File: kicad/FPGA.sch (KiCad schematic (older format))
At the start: 43 parts, among them U11 tx176, U3 MCP4725, X1 Stiftleiste_2x10Pm_R2.54

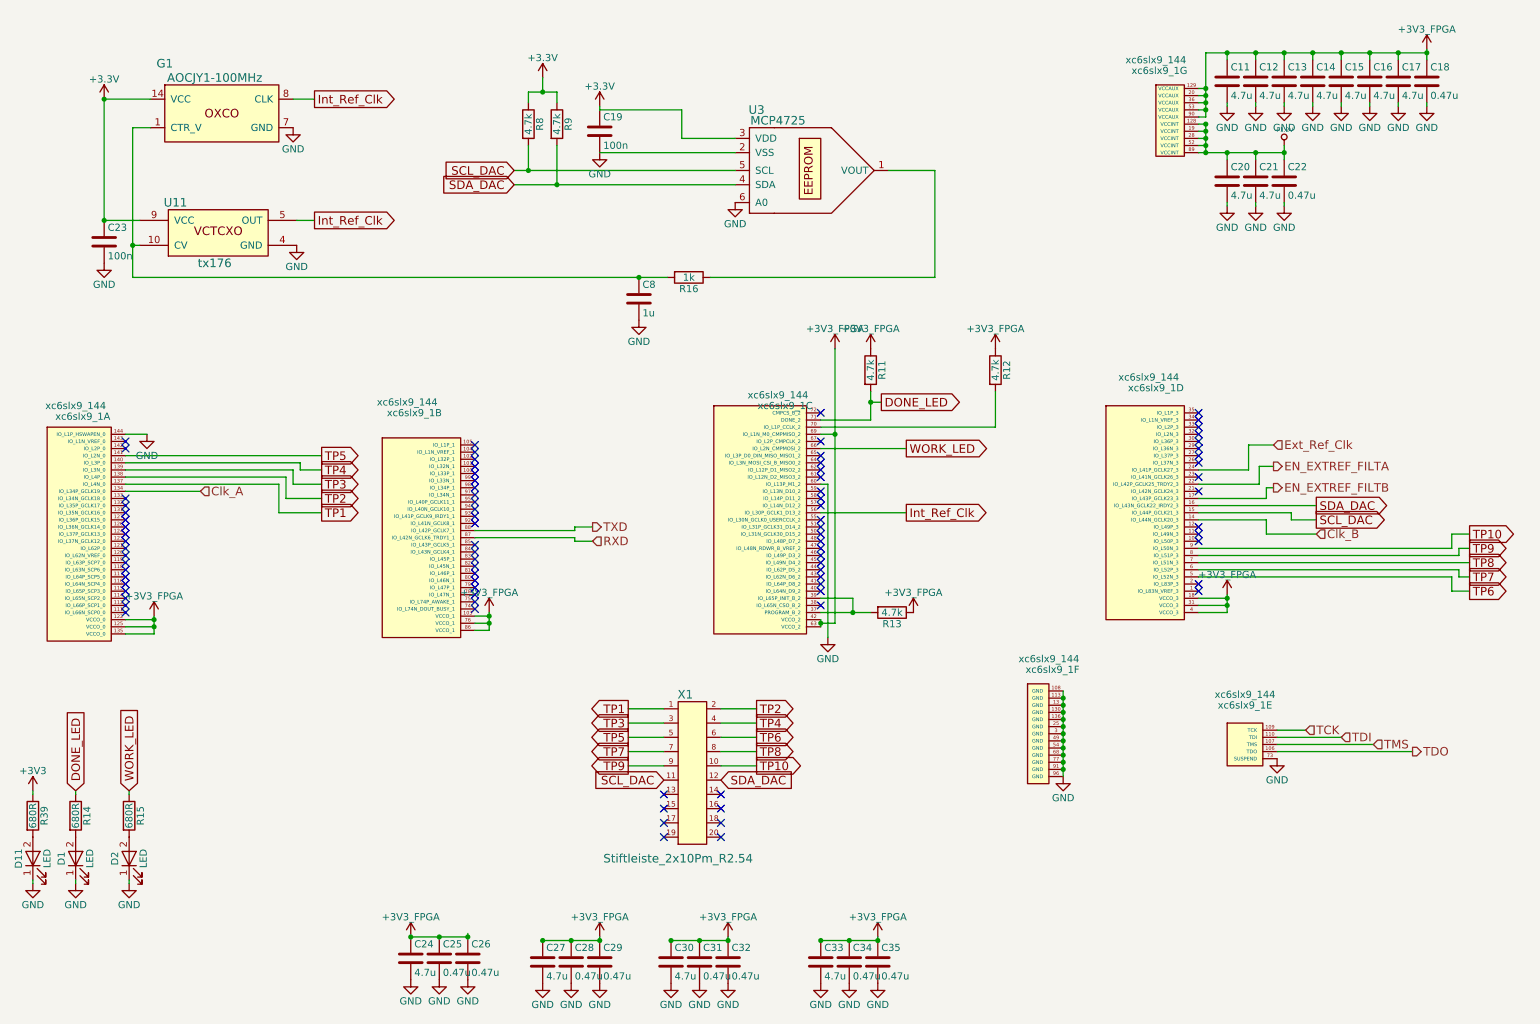
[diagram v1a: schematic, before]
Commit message: some small schematic and layout changes [completed]
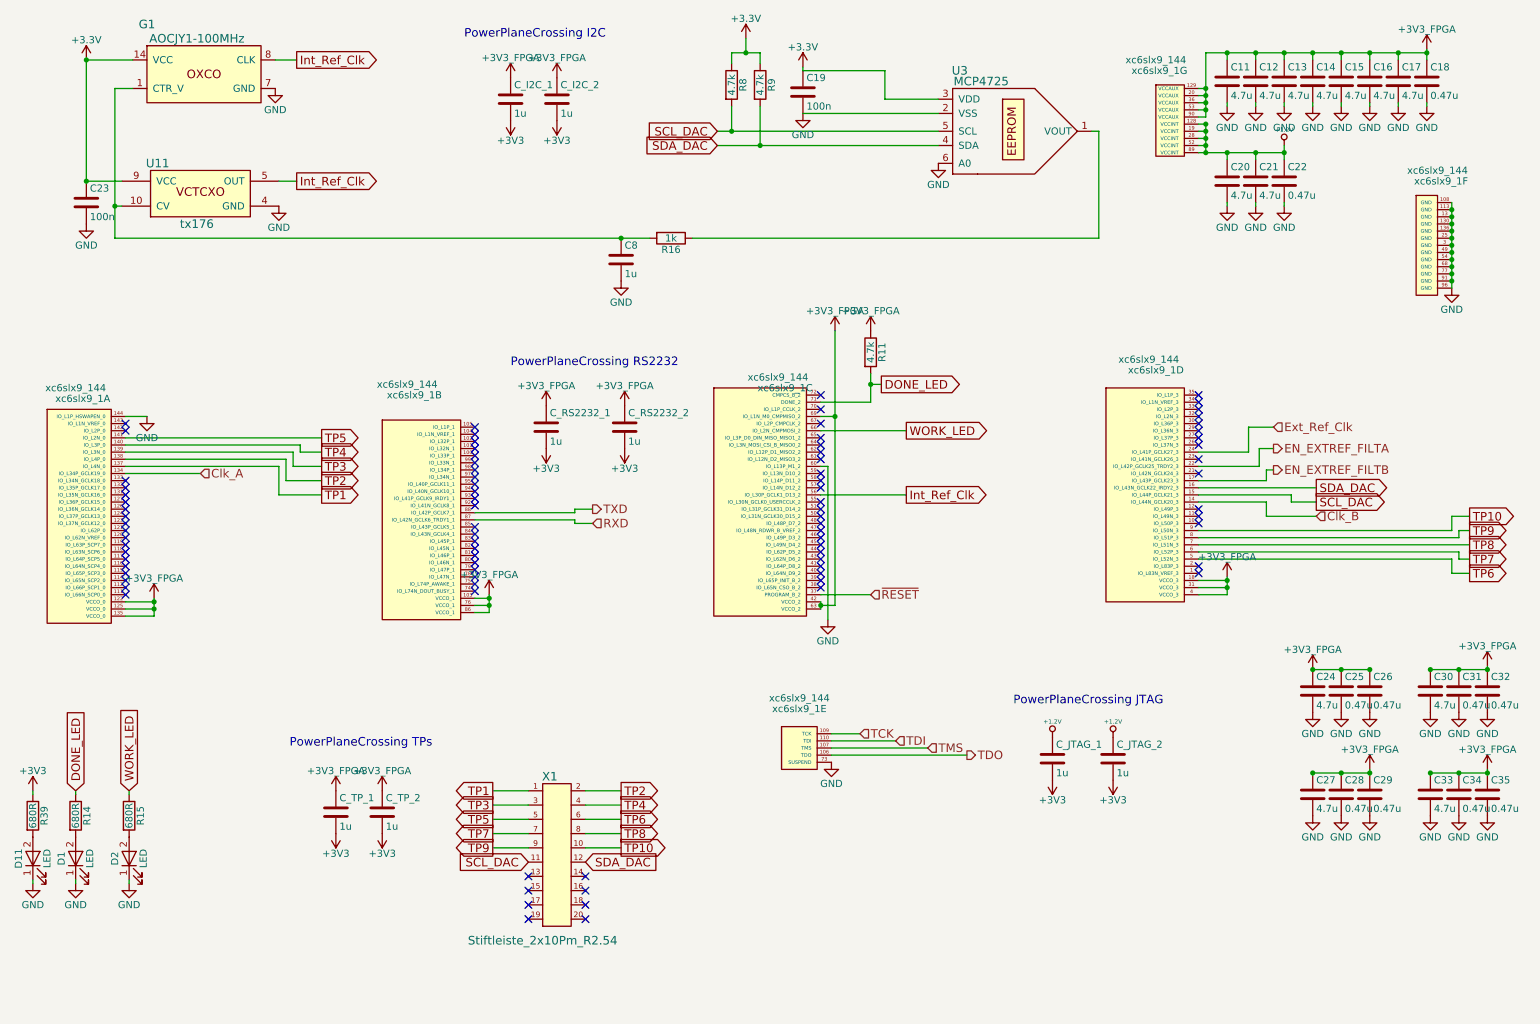
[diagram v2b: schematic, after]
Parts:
- removed R12, R13: 4.7k, Resistors_SMD:R_0603_HandSoldering, symbol R
- added C_I2C_1, C_I2C_2, C_JTAG_1, C_JTAG_2, C_RS2232_1, C_RS2232_2, C_TP_1, C_TP_2: 1u, Capacitors_SMD:C_0603_HandSoldering, symbol C
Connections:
- net +1.2V: now also C_JTAG_1.1, C_JTAG_2.1
- net +3V3: now also C_I2C_1.2, C_I2C_2.2, C_JTAG_1.2, C_JTAG_2.2, C_RS2232_1.2, C_RS2232_2.2, C_TP_1.2, C_TP_2.2
- net +3V3_FPGA: now also C_I2C_1.1, C_I2C_2.1, C_RS2232_1.1, C_RS2232_2.1, C_TP_1.1, C_TP_2.1
- net at xc6slx9_1.39 (IO_L65P_INIT_B_2): no longer xc6slx9_1.37 (PROGRAM_B_2)
- new net ~RESET: xc6slx9_1.37 (PROGRAM_B_2)
- no-connect marks 85 -> 87
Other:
- note added: "PowerPlaneCrossing I2C\n\n"
- note added: "PowerPlaneCrossing JTAG\n\n"
- note added: "PowerPlaneCrossing RS2232\n\n\n"
- note added: "PowerPlaneCrossing TPs\n"
- moved on the sheet: C19, C23, C24, C25, C26, C27, C28, C29, C30, C31, C32, C33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
